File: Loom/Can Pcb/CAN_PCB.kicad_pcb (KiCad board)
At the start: 2 copper layers, 129.5 x 87.9 mm, 33 parts, among them J1 Conn_01x02, J12 Conn_01x03, J15 Conn_01x03, J16 Conn_01x03, J2 Conn_01x05_Pin, J4 Conn_01x02, J5 Conn_01x03, U2 MCP2551-I-P, U4 TL780-05KCS, Y1 Crystal

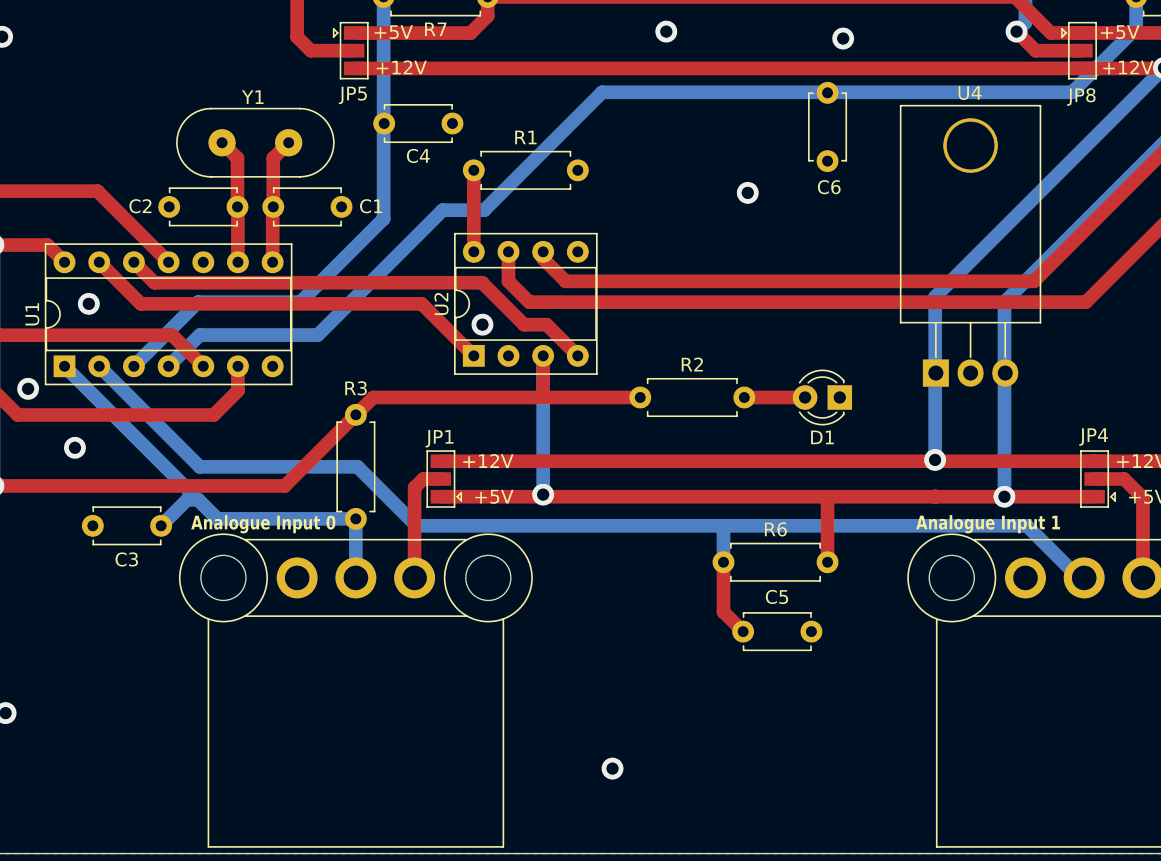
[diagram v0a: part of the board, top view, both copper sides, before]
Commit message: Revert "Merge branch 'CAN_PCB' of https://github.com/Full-Blue-Racing/FBR24-Electronics into CAN_PCB"
This reverts commit f7426b5fd5c3026a458d075125f69338a8895489, reversing
changes made to b85a40d8a8d15d08b24989522968470fc8db4cd4.
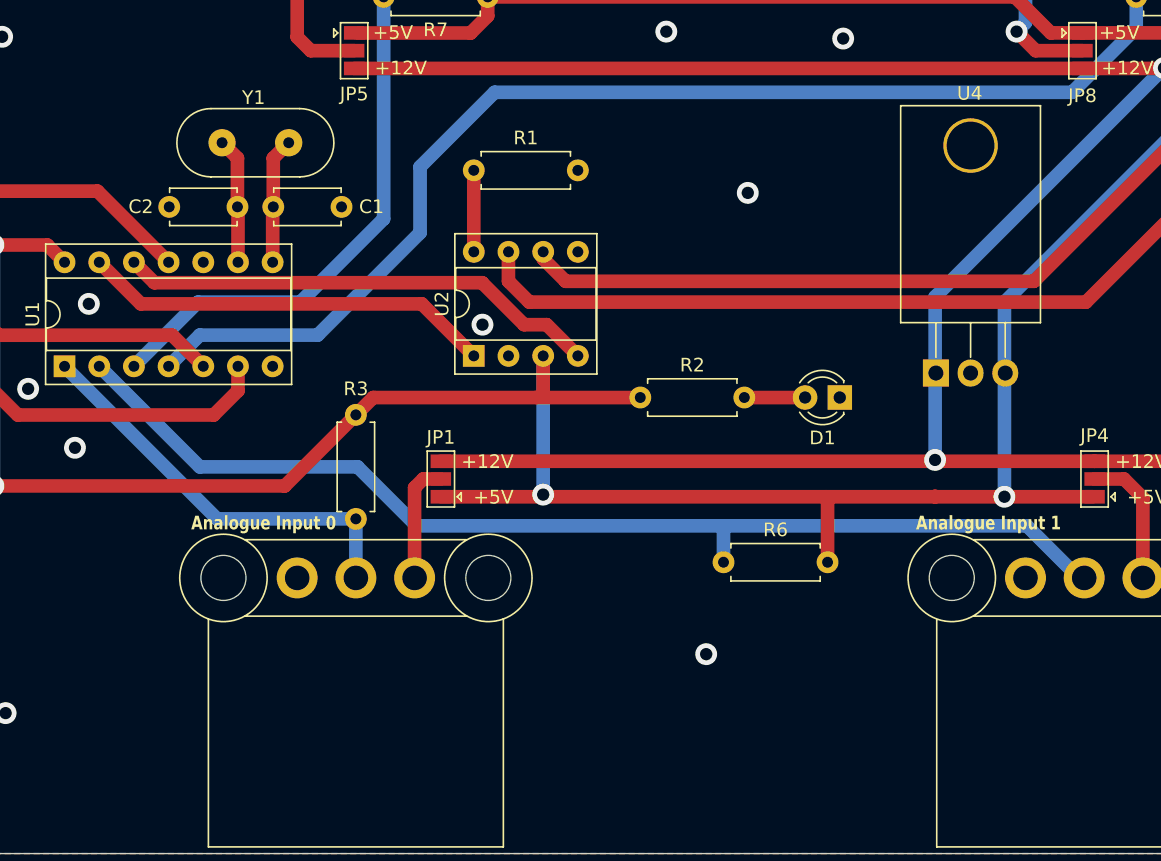
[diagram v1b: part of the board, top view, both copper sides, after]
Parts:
- removed C3, C4, C5, C6: C, Capacitor_THT:C_Disc_D4.7mm_W2.5mm_P5.00mm
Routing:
- net /AN1: track 87.1 -> 81.4 mm
- net /AN0: track 36.1 -> 30.7 mm
- net /AN3: track 90.3 -> 93.2 mm

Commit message: minor changes
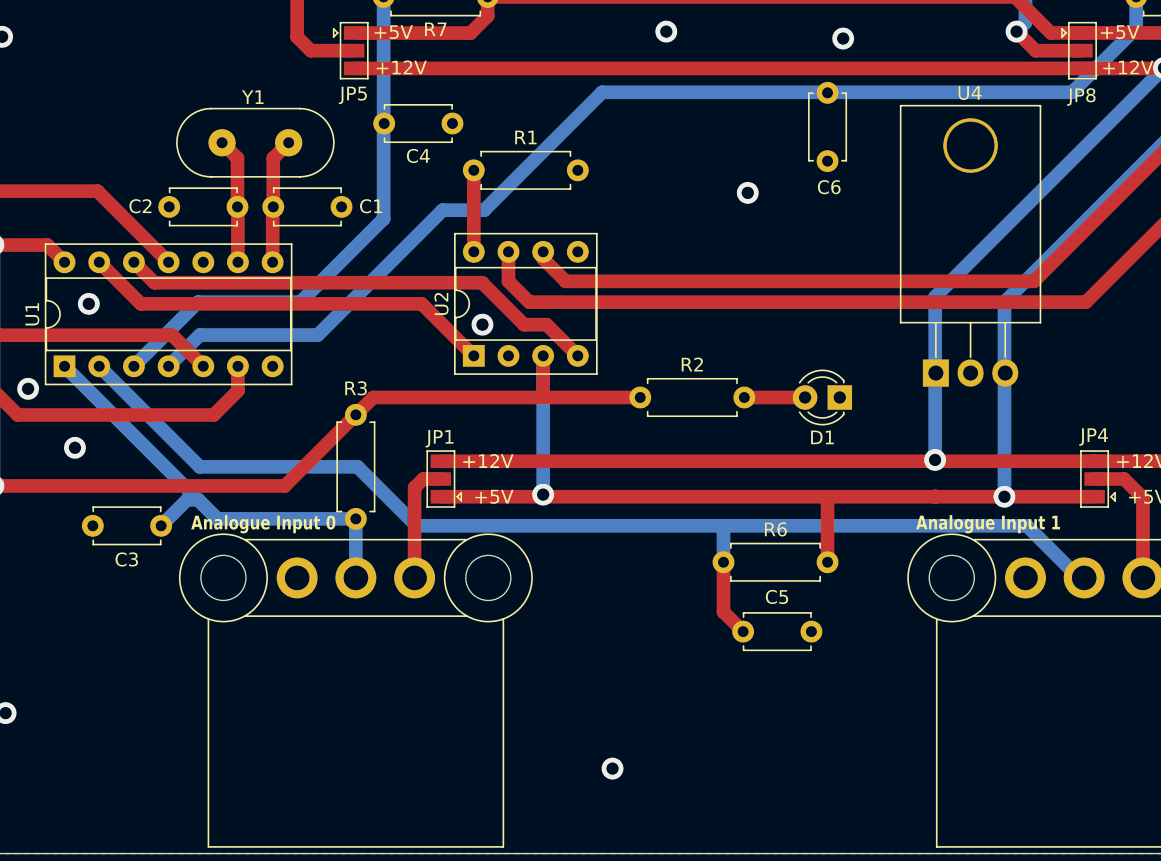
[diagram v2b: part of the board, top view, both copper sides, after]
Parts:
- added C3: C, Capacitor_THT:C_Disc_D4.7mm_W2.5mm_P5.00mm, F.Cu at (116.5, 107.6)
- added C4: C, Capacitor_THT:C_Disc_D4.7mm_W2.5mm_P5.00mm, F.Cu at (132.9, 78.1)
- added C5: C, Capacitor_THT:C_Disc_D4.7mm_W2.5mm_P5.00mm, F.Cu at (159.2, 115.3)
- added C6: C, Capacitor_THT:C_Disc_D4.7mm_W2.5mm_P5.00mm, F.Cu at (165.4, 75.9)
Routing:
- net /AN1: track 81.4 -> 87.1 mm
- net /AN0: track 30.7 -> 36.1 mm
- net /AN3: track 93.2 -> 90.3 mm
